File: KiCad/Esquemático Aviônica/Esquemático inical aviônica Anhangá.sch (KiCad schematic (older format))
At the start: 21 parts, among them J1 Conn_01x06_Female, J2 Conn_01x06_Female, J3 Conn_01x12_Female, J4 Conn_01x12_Female, J5 Screw_Terminal_01x02, J6 Conn_01x06_Male, J7 Screw_Terminal_01x02, J8 Conn_01x02_Female, J9 Conn_01x06_Male, Q1 IRF7403, U1 ME620933

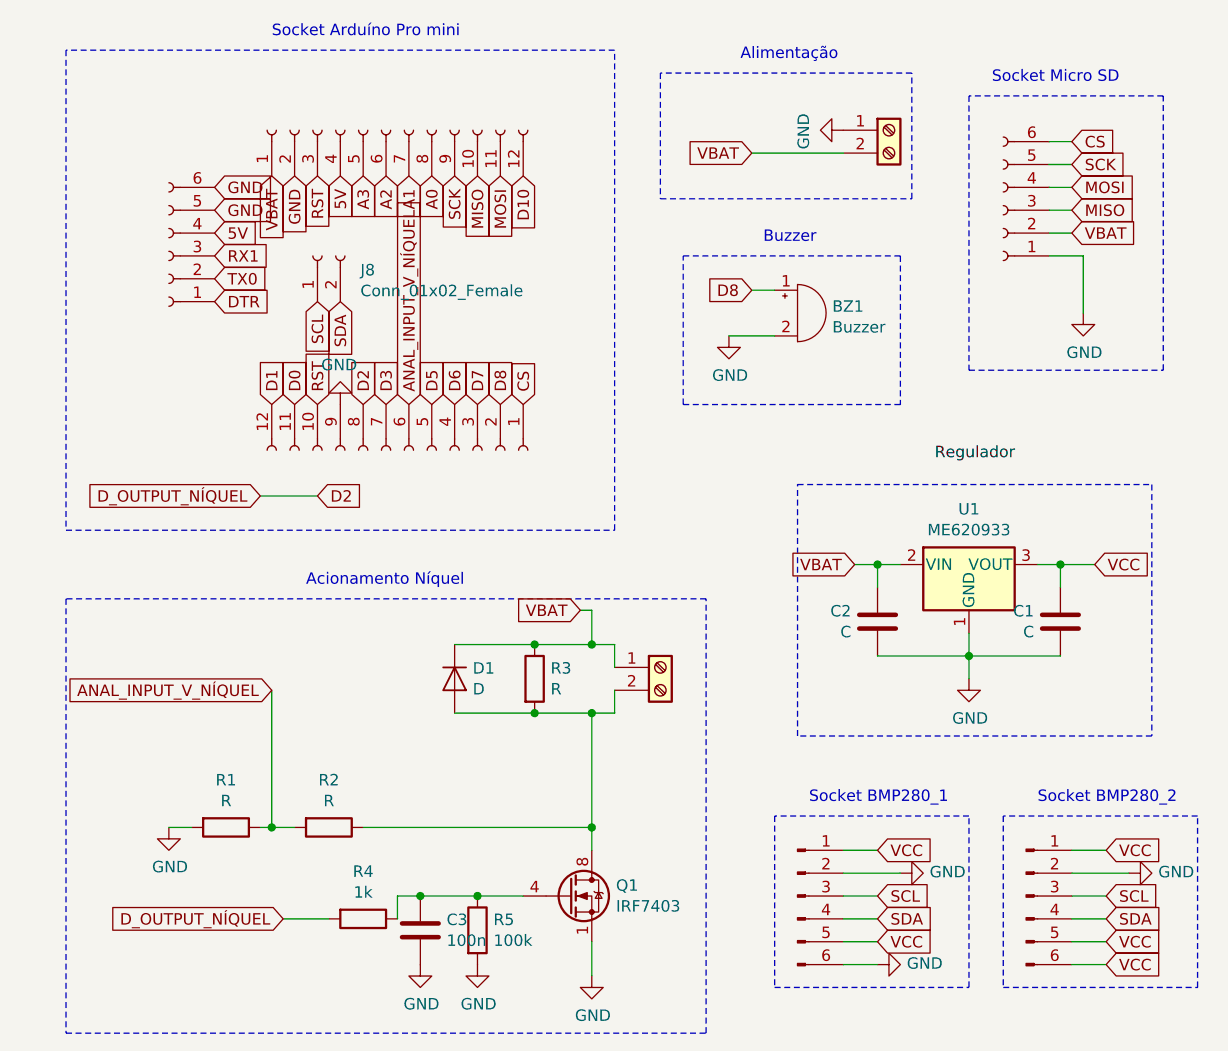
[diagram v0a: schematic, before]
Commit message: PCB Anhangá
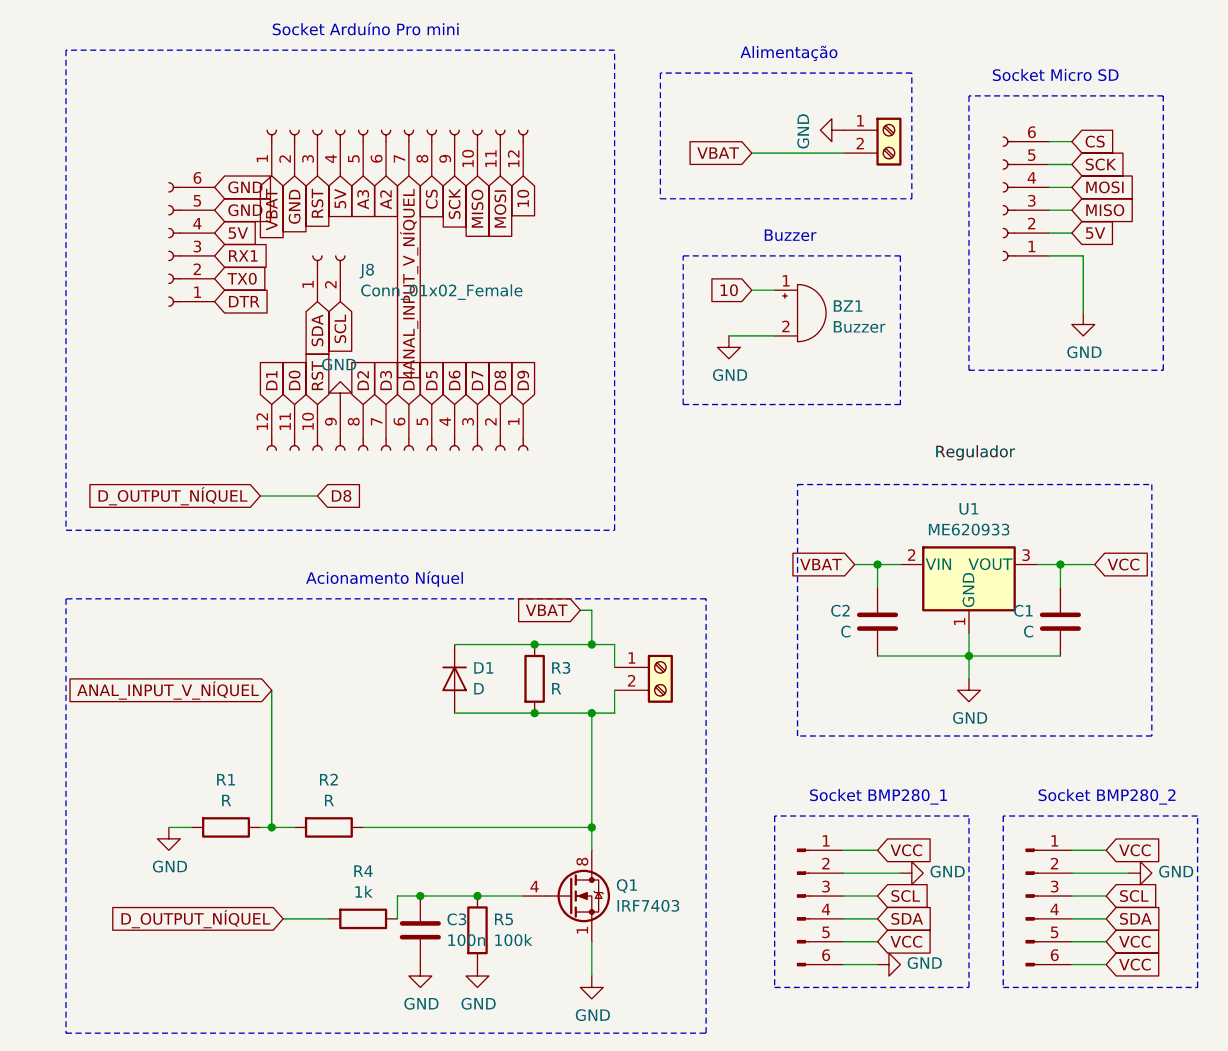
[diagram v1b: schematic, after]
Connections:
- net A0 is gone; now on net CS: J3.8 (Pin_8)
- net A1 is gone; now on net ANAL_INPUT_V_NÍQUEL: J3.7 (Pin_7)
- net 5V: now also J1.2 (Pin_2)
- net ANAL_INPUT_V_NÍQUEL: no longer J4.6 (Pin_6)
- net CS: no longer J4.1 (Pin_1)
- net D2: no longer R4.2
- net D8: now also R4.2; no longer BZ1.1 (-)
- net SCL: now also J8.2 (Pin_2); no longer J8.1 (Pin_1)
- net SDA: now also J8.1 (Pin_1); no longer J8.2 (Pin_2)
- net VBAT: no longer J1.2 (Pin_2)
- net D10 renamed 10
- net 10: now also BZ1.1 (-)
- new net D4: J4.6 (Pin_6)
- new net D9: J4.1 (Pin_1)
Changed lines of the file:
@@
 EESchema Schematic File Version 4
-LIBS:Esquemático inical aviônica Anhangá-cache
 EELAYER 30 0
 EELAYER END
@@
 Text GLabel 2100 3200 2    50   Input ~ 0
 5V
-Text GLabel 2950 2950 3    50   Input ~ 0
-A1
-Text GLabel 3450 3950 1    50   Input ~ 0
-CS
+Text GLabel 3450 2950 3    50   Input ~ 0
+10
 Text GLabel 3150 2950 3    50   Input ~ 0
 SCK
@@
 VBAT
 Text GLabel 5850 3200 2    50   Input ~ 0
-VBAT
+5V
 Wire Notes Line
 	1450 2400 1450 4500
@@
 Text GLabel 2550 3950 1    50   Input ~ 0
 RST
-Text GLabel 2950 3950 1    50   Input ~ 0
+Text GLabel 2950 2950 3    50   Input ~ 0
 ANAL_INPUT_V_NÍQUEL
 Text GLabel 3250 3950 1    50   Input ~ 0
@@
 Text GLabel 2550 2950 3    50   Input ~ 0
 RST
-Text GLabel 3450 2950 3    50   Input ~ 0
-D10
+Text GLabel 3450 3950 1    50   Input ~ 0
+D9
 Wire Notes Line
 	4650 4300 6200 4300
@@
 Text GLabel 2300 4350 0    50   Input ~ 0
 D_OUTPUT_NÍQUEL
-Text GLabel 2550 4350 2    50   Input ~ 0
-D2
 Text GLabel 3350 3950 1    50   Input ~ 0
 D8
 Text GLabel 4450 3450 0    50   Input ~ 0
-D8
+10
 Wire Wire Line
 	2300 4350 2550 4350
@@
 	0    -1   -1   0
 $EndComp
+Text GLabel 2550 3500 3    50   Input ~ 0
+SDA
 Text GLabel 2650 3500 3    50   Input ~ 0
-SDA
-Text GLabel 2550 3500 3    50   Input ~ 0
 SCL
-Text GLabel 3050 2950 3    50   Input ~ 0
-A0
 $Comp
 L Connector:Conn_01x02_Female J8
@@
 	1    0    0    -1
 $EndComp
+Text GLabel 2950 3950 1    50   Input ~ 0
+D4
+Text GLabel 3050 2950 3    50   Input ~ 0
+CS
+Text GLabel 2550 4350 2    50   Input ~ 0
+D8
 $EndSCHEMATC
